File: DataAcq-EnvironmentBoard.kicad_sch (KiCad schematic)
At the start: 25 parts, among them J1 CAN Output, J2 CAN Input, U1 SHT45, U2 FS3000-1005, U3 LMT87DCK, U4 Daughterboard Connector

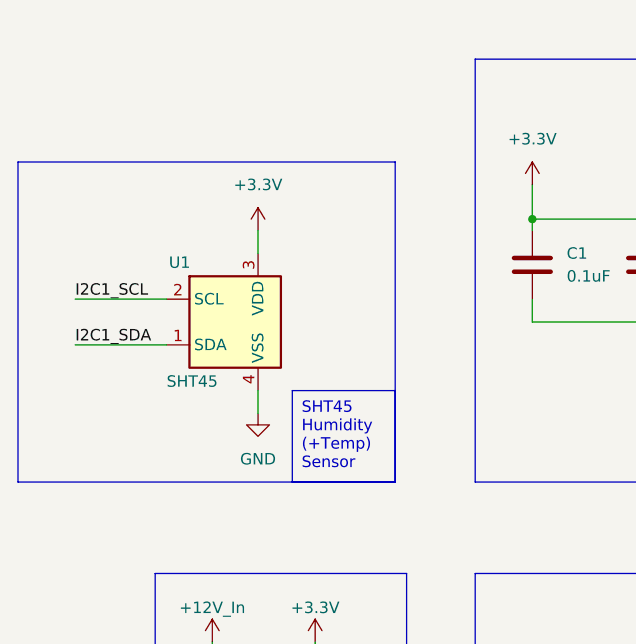
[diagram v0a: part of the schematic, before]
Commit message: cap
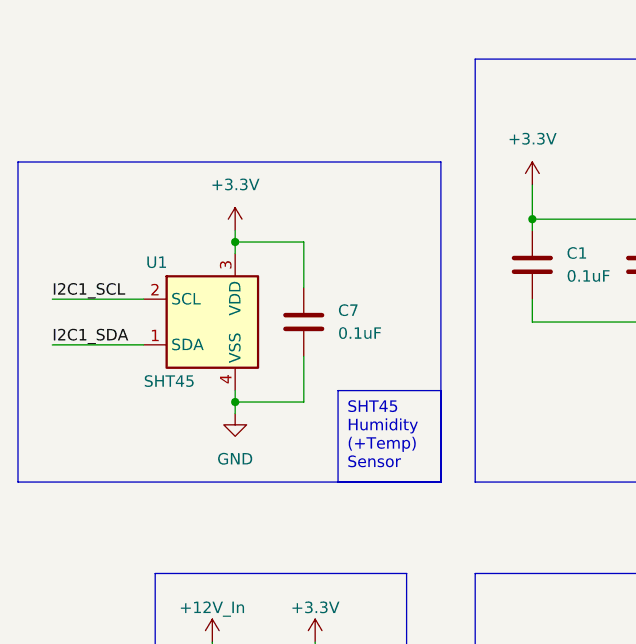
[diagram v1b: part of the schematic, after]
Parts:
- added C7: 0.1uF, Capacitor_SMD:C_0805_2012Metric, symbol Device:C
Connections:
- net +3.3V: now also C7.1
- net GND: now also C7.2
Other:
- moved on the sheet: U1
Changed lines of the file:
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@@
 	)
 	(junction
+		(at 52.07 78.74)
+		(diameter 0)
+		(color 0 0 0 0)
+	)
+	(junction
 		(at 215.9 49.53)
 		(diameter 0)
 		(color 0 0 0 0)
 	)
+	(junction
+		(at 52.07 60.96)
+		(diameter 0)
+		(color 0 0 0 0)
+	)
 	(no_connect
 		(at 142.24 137.16)
@@
 	(wire
 		(pts
+			(xy 52.07 60.96) (xy 52.07 62.23)
+		)
+		(stroke
+			(width 0)
+			(type default)
+		)
+	)
+	(wire
+		(pts
 			(xy 172.72 116.84) (xy 185.42 116.84)
 		)
@@
 	(wire
 		(pts
-			(xy 34.29 72.39) (xy 44.45 72.39)
+			(xy 31.75 72.39) (xy 41.91 72.39)
 		)
 		(stroke
@@
 	(wire
 		(pts
-			(xy 54.61 77.47) (xy 54.61 80.01)
+			(xy 52.07 77.47) (xy 52.07 78.74)
+		)
+		(stroke
+			(width 0)
+			(type default)
+		)
+	)
+	(wire
+		(pts
+			(xy 59.69 78.74) (xy 52.07 78.74)
 		)
 		(stroke
@@
 	(wire
 		(pts
+			(xy 59.69 73.66) (xy 59.69 78.74)
+		)
+		(stroke
+			(width 0)
+			(type default)
+		)
+	)
+	(wire
+		(pts
+			(xy 59.69 66.04) (xy 59.69 60.96)
+		)
+		(stroke
+			(width 0)
+			(type default)
+		)
+	)
+	(wire
+		(pts
 			(xy 250.19 62.23) (xy 261.62 62.23)
 		)
@@
 	(wire
 		(pts
-			(xy 34.29 67.31) (xy 44.45 67.31)
+			(xy 31.75 67.31) (xy 41.91 67.31)
 		)
 		(stroke
@@
 	(wire
 		(pts
+			(xy 59.69 60.96) (xy 52.07 60.96)
+		)
+		(stroke
+			(width 0)
+			(type default)
+		)
+	)
+	(wire
+		(pts
 			(xy 97.79 55.88) (xy 123.19 55.88)
 		)
@@
 	(wire
 		(pts
+			(xy 52.07 78.74) (xy 52.07 80.01)
+		)
+		(stroke
+			(width 0)
+			(type default)
+		)
+	)
+	(wire
+		(pts
 			(xy 218.44 49.53) (xy 218.44 54.61)
 		)
@@
 	(wire
 		(pts
-			(xy 54.61 59.69) (xy 54.61 62.23)
+			(xy 52.07 59.69) (xy 52.07 60.96)
 		)
 		(stroke
@@
 	(rectangle
 		(start 27.94 52.07)
-		(end 69.85 87.63)
+		(end 74.93 87.63)
 		(stroke
 			(width 0)
@@
 	(text_box "SHT45 Humidity (+Temp) Sensor\n"
 		(exclude_from_sim no)
-		(at 58.42 77.47 0)
+		(at 63.5 77.47 0)
 		(size 11.43 10.16)
 		(stroke
@@
 	)
 	(label "I2C1_SCL"
-		(at 34.29 67.31 0)
+		(at 31.75 67.31 0)
 		(fields_autoplaced yes)
 		(effects
@@
 	)
 	(label "I2C1_SDA"
-		(at 34.29 72.39 0)
+		(at 31.75 72.39 0)
 		(fields_autoplaced yes)
 		(effects
@@
 	(symbol
 		(lib_id "power:GND")
-		(at 54.61 80.01 0)
+		(at 52.07 80.01 0)
 		(unit 1)
 		(exclude_from_sim no)
@@
 		(fields_autoplaced yes)
 		(property "Reference" "#PWR01"
-			(at 54.61 86.36 0)
+			(at 52.07 86.36 0)
 			(effects
 				(font
@@
 		)
 		(property "Value" "GND"
-			(at 54.61 85.09 0)
+			(at 52.07 85.09 0)
 			(effects
 				(font
@@
 		)
 		(property "Footprint" ""
-			(at 54.61 80.01 0)
+			(at 52.07 80.01 0)
 			(effects
 				(font
@@
 		)
 		(property "Datasheet" ""
-			(at 54.61 80.01 0)
+			(at 52.07 80.01 0)
 			(effects
 				(font
@@
 		)
 		(property "Description" "Power symbol creates a global label with name \"GND\" , ground"
-			(at 54.61 80.01 0)
+			(at 52.07 80.01 0)
 			(effects
 				(font
@@
 	(symbol
 		(lib_id "Sensor_Humidity:SHT4x")
-		(at 52.07 69.85 0)
+		(at 49.53 69.85 0)
 		(unit 1)
 		(exclude_from_sim no)
@@
 		(dnp no)
 		(property "Reference" "U1"
-			(at 44.704 63.246 0)
+			(at 42.164 63.246 0)
 			(effects
 				(font
@@
 		)
 		(property "Value" "SHT45"
-			(at 44.45 76.454 0)
+			(at 41.91 76.454 0)
 			(effects
 				(font
@@
 		)
 		(property "Footprint" "Sensor_Humidity:Sensirion_DFN-4_1.5x1.5mm_P0.8mm_SHT4x_NoCentralPad"
-			(at 55.88 76.2 0)
+			(at 53.34 76.2 0)
 			(effects
 				(font
@@
 		)
 		(property "Datasheet" "https://sensirion.com/media/documents/33FD6951/624C4357/Datasheet_SHT4x.pdf"
-			(at 55.88 78.74 0)
+			(at 53.34 78.74 0)
 			(effects
 				(font
@@
 		)
 		(property "Description" "Digital Humidity and Temperature Sensor, +/-1%RH, +/-0.1degC, I2C, 1.08-3.6V, 16bit, DFN-4"
-			(at 52.07 69.85 0)
+			(at 49.53 69.85 0)
 			(effects
 				(font
@@
 		)
 		(property "P/N" "SHT45-AD1B-R3 "
-			(at 52.07 69.85 0)
+			(at 49.53 69.85 0)
 			(effects
 				(font
@@
 	(symbol
 		(lib_id "power:+3.3V")
-		(at 54.61 59.69 0)
+		(at 52.07 59.69 0)
 		(unit 1)
 		(exclude_from_sim no)
@@
 		(fields_autoplaced yes)
 		(property "Reference" "#PWR02"
-			(at 54.61 63.5 0)
+			(at 52.07 63.5 0)
 			(effects
 				(font
@@
 		)
 		(property "Value" "+3.3V"
-			(at 54.61 54.61 0)
+			(at 52.07 54.61 0)
 			(effects
 				(font
@@
 		)
 		(property "Footprint" ""
-			(at 54.61 59.69 0)
+			(at 52.07 59.69 0)
 			(effects
 				(font
@@
 		)
 		(property "Datasheet" ""
-			(at 54.61 59.69 0)
+			(at 52.07 59.69 0)
 			(effects
 				(font
@@
 		)
 		(property "Description" "Power symbol creates a global label with name \"+3.3V\""
-			(at 54.61 59.69 0)
+			(at 52.07 59.69 0)
 			(effects
 				(font
@@
 					(unit 1)
 				)
+			)
+		)
+	)
+	(symbol
+		(lib_id "Device:C")
+		(at 59.69 69.85 0)
+		(unit 1)
+		(exclude_from_sim no)
+		(in_bom yes)
+		(on_board yes)
+		(dnp no)
+		(fields_autoplaced yes)
+		(property "Reference" "C7"
+			(at 63.5 68.5799 0)
+			(effects
+				(font
+					(size 1.27 1.27)
+				)
+				(justify left)
+			)
+		)
+		(property "Value" "0.1uF"
+			(at 63.5 71.1199 0)
+			(effects
+				(font
+					(size 1.27 1.27)
+				)
+				(justify left)
+			)
+		)
+		(property "Footprint" "Capacitor_SMD:C_0805_2012Metric"
+			(at 60.6552 73.66 0)
+			(effects
+				(font
+					(size 1.27 1.27)
+				)
+				(hide yes)
+			)
+		)
+		(property "Datasheet" "~"
+			(at 59.69 69.85 0)
+			(effects
+				(font
+					(size 1.27 1.27)
+				)
+				(hide yes)
+			)
+		)
+		(property "Description" "Unpolarized capacitor"
+			(at 59.69 69.85 0)
+			(effects
+				(font
+					(size 1.27 1.27)
+				)
+				(hide yes)
+			)
+		)
+		(property "P/N" "C0805C104M5RACTU"
+			(at 59.69 69.85 0)
+			(effects
+				(font
+					(size 1.27 1.27)
+				)
+				(hide yes)
+			)
+		)
+		(pin "2"
+		)
+		(pin "1"
+		)
+		(instances
+			(project "DataAcq-EnvironmentBoard"
+				(path "/bc5fb1f8-c603-414b-89d1-18cc156ddb66"
+					(reference "C7")
+					(unit 1)
+				)
